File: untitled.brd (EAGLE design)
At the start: 59.4 x 57.8 mm, 25 parts

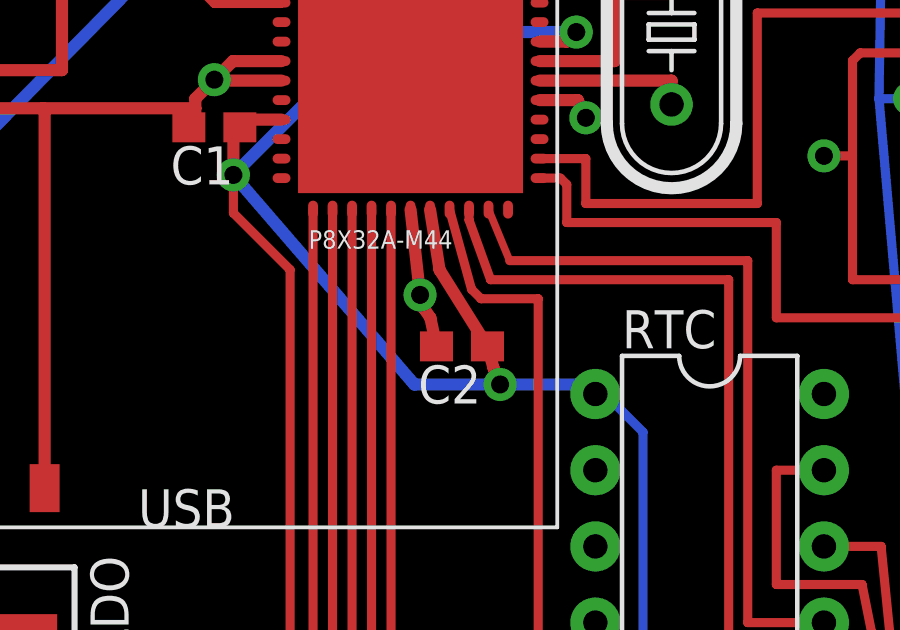
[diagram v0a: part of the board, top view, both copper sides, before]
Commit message: made the traces look better
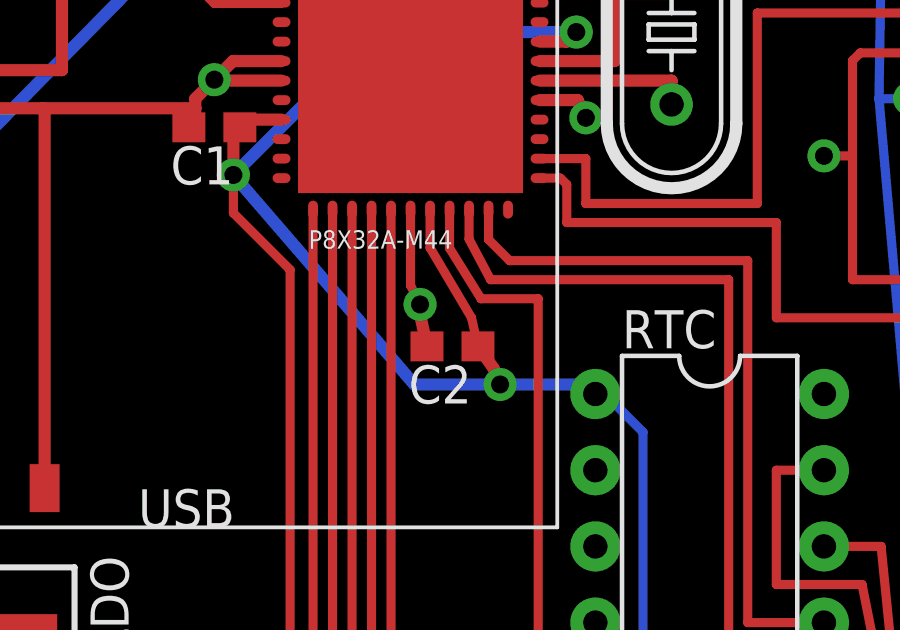
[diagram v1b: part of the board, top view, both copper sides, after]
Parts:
- moved C2 0.32 mm to (56.2, 34.0)
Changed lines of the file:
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@@
 <element name="U$2" library="SparkFun" package="LCC36" value="HMC6343A" x="86.995" y="23.495"/>
 <element name="C1" library="rcl" package="C0603" value="" x="48.26" y="41.275" rot="R180"/>
-<element name="C2" library="rcl" package="C0603" value="" x="56.515" y="33.9725" rot="R180"/>
+<element name="C2" library="rcl" package="C0603" value="" x="56.1975" y="33.9725" rot="R180"/>
 <element name="C3" library="rcl" package="C0603" value="" x="53.6575" y="51.1175" rot="R90"/>
 <element name="C4" library="SparkFun" package="0603" value="" x="79.6925" y="25.0825" rot="R90"/>
@@
 <wire x1="66.04" y1="36.83" x2="66.04" y2="24.765" width="0.3048" layer="1"/>
 <wire x1="66.04" y1="24.765" x2="68.58" y2="24.765" width="0.3048" layer="1"/>
-<wire x1="57.4" y1="38.5313" x2="58.1025" y2="36.83" width="0.254" layer="1"/>
+<wire x1="57.4" y1="38.5313" x2="57.4" y2="37.5325" width="0.3048" layer="1"/>
+<wire x1="57.4" y1="37.5325" x2="58.1025" y2="36.83" width="0.3048" layer="1"/>
 </signal>
 <signal name="N$6">
@@
 <wire x1="70.8025" y1="24.13" x2="70.485" y2="27.305" width="0.3048" layer="1"/>
 <wire x1="70.485" y1="27.305" x2="68.58" y2="27.305" width="0.3048" layer="1"/>
-<wire x1="56.1" y1="38.5313" x2="56.8325" y2="35.8775" width="0.3048" layer="1"/>
-<wire x1="56.8325" y1="35.8775" x2="57.15" y2="35.56" width="0.3048" layer="1"/>
 <wire x1="57.15" y1="35.56" x2="59.055" y2="35.56" width="0.3048" layer="1"/>
+<wire x1="56.1" y1="38.5313" x2="56.1" y2="37.245" width="0.3048" layer="1"/>
+<wire x1="56.1" y1="37.245" x2="57.15" y2="35.56" width="0.3048" layer="1"/>
 </signal>
 <signal name="N$8">
@@
 <wire x1="66.9925" y1="26.035" x2="66.9925" y2="29.845" width="0.3048" layer="1"/>
 <wire x1="66.9925" y1="29.845" x2="68.58" y2="29.845" width="0.3048" layer="1"/>
-<wire x1="56.75" y1="38.5313" x2="56.75" y2="38.1825" width="0.3048" layer="1"/>
-<wire x1="56.75" y1="38.1825" x2="57.4675" y2="36.195" width="0.3048" layer="1"/>
+<wire x1="56.75" y1="38.5313" x2="56.75" y2="37.5475" width="0.3048" layer="1"/>
+<wire x1="56.75" y1="37.5475" x2="57.4675" y2="36.195" width="0.3048" layer="1"/>
 </signal>
 <signal name="SCL">
@@
 <vertex x="33.655" y="10.16"/>
 </polygon>
-<wire x1="54.8" y1="38.5313" x2="55.1175" y2="35.6875" width="0.4064" layer="1"/>
-<wire x1="55.245" y1="35.2425" x2="55.46" y2="34.925" width="0.4064" layer="1"/>
-<wire x1="55.46" y1="34.925" x2="55.665" y2="33.9725" width="0.4064" layer="1"/>
+<wire x1="55.1425" y1="34.925" x2="55.3475" y2="33.9725" width="0.4064" layer="1"/>
 <wire x1="54.8" y1="47.1313" x2="54.8" y2="52.07" width="0.4064" layer="1"/>
 <wire x1="54.8" y1="52.07" x2="54.4825" y2="53.4675" width="0.4064" layer="1"/>
@@
 <via x="48.26" y="42.8625" extent="1-16" drill="0.6"/>
 <via x="54.4825" y="53.4675" extent="1-16" drill="0.6"/>
-<via x="55.1175" y="35.6875" extent="1-16" drill="0.6"/>
+<via x="55.1175" y="35.37" extent="1-16" drill="0.6"/>
 <wire x1="59.1" y1="42.1813" x2="60.3712" y2="42.1813" width="0.4064" layer="1"/>
 <wire x1="60.3712" y1="42.1813" x2="60.6425" y2="41.5925" width="0.4064" layer="1"/>
 <via x="60.6425" y="41.5925" extent="1-16" drill="0.6"/>
-<wire x1="55.245" y1="35.2425" x2="55.1175" y2="35.6875" width="0.4064" layer="1"/>
 <wire x1="89.395" y1="27.895" x2="89.395" y2="25.54" width="0.3048" layer="1"/>
 <wire x1="89.395" y1="25.54" x2="89.84" y2="25.095" width="0.3048" layer="1"/>
@@
 <wire x1="42.545" y1="41.91" x2="47.625" y2="41.91" width="0.4064" layer="1"/>
 <wire x1="42.6025" y1="41.8525" x2="42.545" y2="41.91" width="0.4064" layer="1" curve="90"/>
+<wire x1="54.8" y1="38.5313" x2="54.8" y2="36.005" width="0.3048" layer="1"/>
+<wire x1="54.8" y1="36.005" x2="55.1175" y2="35.37" width="0.3048" layer="1"/>
+<wire x1="55.1425" y1="34.925" x2="55.1175" y2="34.95" width="0.3048" layer="1" curve="-90"/>
+<wire x1="55.1175" y1="34.95" x2="55.1175" y2="35.37" width="0.3048" layer="1"/>
+<wire x1="81.915" y1="60.325" x2="89.535" y2="60.325" width="0" layer="19" extent="1-1"/>
+<wire x1="81.915" y1="62.865" x2="81.915" y2="60.325" width="0" layer="19" extent="1-1"/>
+<wire x1="81.915" y1="57.785" x2="81.915" y2="60.325" width="0" layer="19" extent="1-1"/>
+<wire x1="81.915" y1="55.245" x2="81.915" y2="57.785" width="0" layer="19" extent="1-1"/>
+<wire x1="74.05" y1="43.755" x2="81.915" y2="55.245" width="0" layer="19" extent="1-1"/>
+<wire x1="80.3275" y1="30.7975" x2="75.2475" y2="36.195" width="0" layer="19" extent="1-1"/>
+<wire x1="60.6425" y1="41.5925" x2="68.58" y2="40.3225" width="0" layer="19" extent="1-1"/>
+<wire x1="54.8" y1="38.5313" x2="59.1" y2="42.1813" width="0" layer="19" extent="1-1"/>
+<wire x1="50.5" y1="42.8313" x2="54.8" y2="38.5313" width="0" layer="19" extent="1-1"/>
+<wire x1="54.8" y1="47.1313" x2="50.5" y2="43.4813" width="0" layer="19" extent="1-1"/>
+<wire x1="60.325" y1="59.69" x2="54.4825" y2="53.4675" width="0" layer="19" extent="1-1"/>
+<wire x1="57.785" y1="64.77" x2="60.325" y2="59.69" width="0" layer="19" extent="1-1"/>
+<wire x1="60.96" y1="24.765" x2="55.3475" y2="33.9725" width="0" layer="19" extent="1-1"/>
+<wire x1="70.77" y1="13.51" x2="75.2475" y2="27.6225" width="0" layer="19" extent="1-1"/>
+<wire x1="40.64" y1="66.04" x2="57.785" y2="64.77" width="0" layer="19" extent="1-1"/>
+<wire x1="36.83" y1="62.96" x2="40.64" y2="66.04" width="0" layer="19" extent="1-1"/>
 </signal>
 <signal name="+5V">
@@
 <wire x1="48.895" y1="39.6875" x2="48.895" y2="41.06" width="0.4064" layer="1"/>
 <wire x1="48.895" y1="41.06" x2="49.11" y2="41.275" width="0.4064" layer="1"/>
-<wire x1="57.365" y1="33.9725" x2="57.57" y2="33.235" width="0.4064" layer="1"/>
+<wire x1="57.0475" y1="33.9725" x2="57.57" y2="33.235" width="0.4064" layer="1"/>
 <wire x1="57.57" y1="33.235" x2="57.785" y2="32.7025" width="0.4064" layer="1"/>
 <via x="57.785" y="32.7025" extent="1-16" drill="0.6"/>
@@
 <wire x1="51.7525" y1="49.8475" x2="52.3875" y2="45.72" width="0.4064" layer="16"/>
 <wire x1="52.3875" y1="45.72" x2="53.6575" y2="44.45" width="0.4064" layer="16"/>
-<wire x1="55.7675" y1="36.5225" x2="57.365" y2="33.9725" width="0.4064" layer="1"/>
 <wire x1="60.96" y1="32.385" x2="60.96" y2="32.7025" width="0.4064" layer="16"/>
 <wire x1="60.96" y1="32.7025" x2="57.785" y2="32.7025" width="0.4064" layer="16"/>
@@
 <wire x1="35.2425" y1="40.64" x2="40.3225" y2="40.64" width="0.4064" layer="1"/>
 <wire x1="40.3225" y1="40.64" x2="40.3225" y2="21.9475" width="0.4064" layer="1"/>
-<wire x1="55.45" y1="38.5313" x2="55.7675" y2="36.5225" width="0.4064" layer="1"/>
+<wire x1="55.45" y1="38.5313" x2="55.45" y2="37.26" width="0.3048" layer="1"/>
+<wire x1="56.515" y1="34.505" x2="57.0475" y2="33.9725" width="0" layer="19" extent="1-16"/>
+<wire x1="55.45" y1="37.26" x2="56.8325" y2="34.925" width="0.3048" layer="1"/>
+<wire x1="56.8325" y1="34.925" x2="57.0475" y2="33.9725" width="0.3048" layer="1"/>
 </signal>
 </signals>
